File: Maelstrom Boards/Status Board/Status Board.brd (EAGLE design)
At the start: 101.6 x 76.2 mm, 32 parts, among them IC1 LM555D, P1 39-30-04?, Q1 310mA/60V/1.6Ω, Q2 310mA/60V/1.6Ω

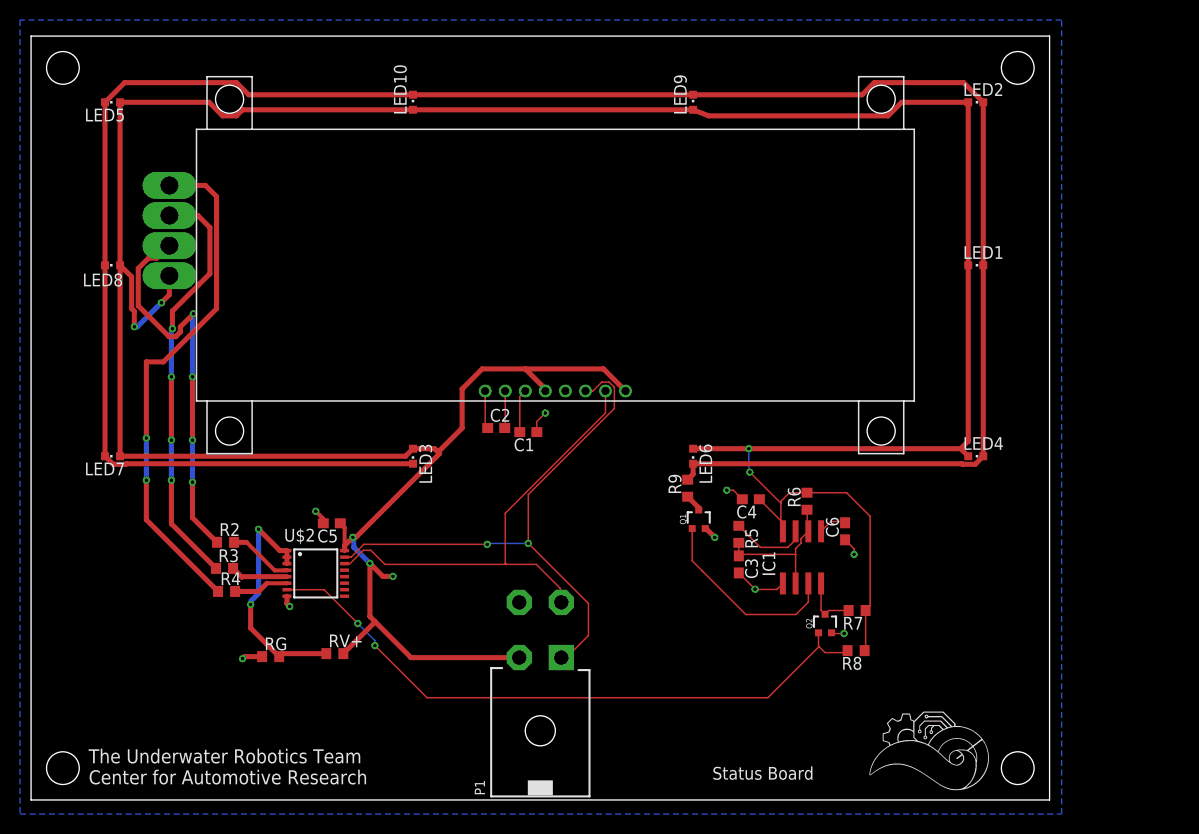
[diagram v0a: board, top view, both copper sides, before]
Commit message: Update Status Board
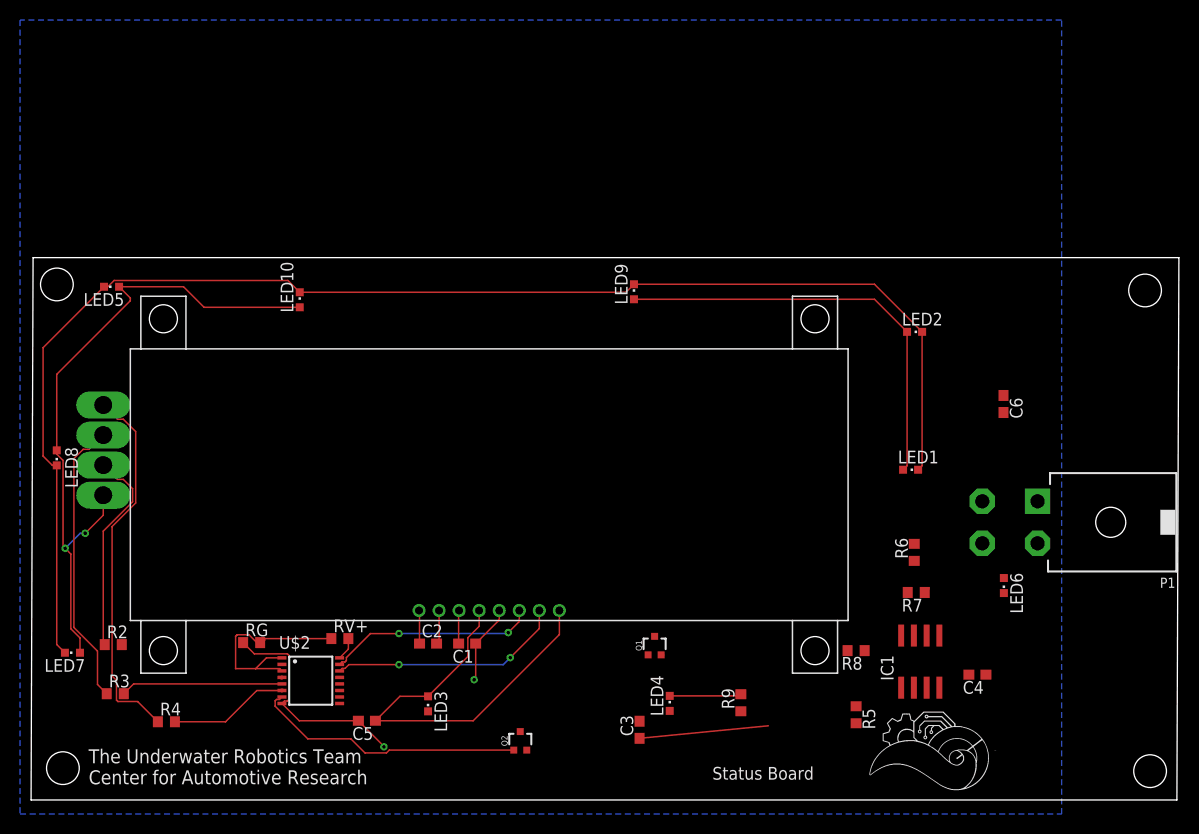
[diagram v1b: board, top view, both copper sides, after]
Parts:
- R5: value 50k -> 100k
- R6: value 100k -> 1k
- moved P1 51.4 mm to (100.4, 27.7), turned to 90 degrees
- moved LED4 39.2 mm to (63.7, 9.63), turned to 0 degrees
- moved LED6 33.6 mm to (97.0, 21.4)
- moved Q2 32.6 mm to (48.8, 5.90)
- moved C4 28.6 mm to (94.4, 12.5)
- moved LED3 24.7 mm to (39.6, 9.59)
- moved LED2 23.7 mm to (88.1, 46.7)
- moved U$1 22.9 mm to (13.2, 14.9)
- moved LED10 22.7 mm to (26.8, 49.9)
- moved C2 22.5 mm to (39.6, 15.6)
- moved R9 22.0 mm to (70.8, 9.70)
- moved C1 22.0 mm to (43.5, 15.6)
- moved R5 21.5 mm to (82.3, 8.50)
- moved LED1 21.4 mm to (87.7, 32.9)
- moved C6 20.3 mm to (97.0, 39.5), turned to 270 degrees
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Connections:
- net +3V3: now also R6.1; no longer R6.2
- net N$10: no longer R6.1
- net N$9: now also R6.2
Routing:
- net +3V3: track 344.8 -> 153.9 mm, vias 7 -> 2
- net N$20: track 223.0 -> 145.9 mm
- net BLINK_ON: track 64.8 -> 27.8 mm, vias 2 -> 0
- net SDA: track 56.8 -> 21.0 mm
- net SCL: track 46.6 -> 23.5 mm, vias 0 -> 2
- net BLINK: track 19.4 -> 0.00 mm
- net N$7: track 39.7 -> 20.7 mm, vias 4 -> 0
- net N$5: track 51.4 -> 37.3 mm, vias 2 -> 0
- net N$1: track 42.0 -> 28.7 mm, vias 4 -> 0
- net GND: track 18.9 -> 30.7 mm, vias 9 -> 2
- net GREEN: track 5.75 -> 16.2 mm
- net N$9: track 7.71 -> 0.83 mm
- net BLUE: track 5.52 -> 12.0 mm
- net RED: track 6.45 -> 0.04 mm
- net BLINK_OFF: track 5.74 -> 0.00 mm
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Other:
- board size 101.6 x 76.2 mm -> 114.5 x 54.1 mm
